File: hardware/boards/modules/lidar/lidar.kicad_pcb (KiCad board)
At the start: 2 copper layers, 70.6 x 66 mm, 33 parts, among them J1 Conn_01x04_Socket, J2 Lidar, J3 Conn_01x03_Socket, J4 Conn_01x03_Socket, J5 Conn_01x03_Socket, J6 Conn_01x03_Socket, J7 Conn_01x05_Socket, J8 Conn_01x04_Socket, Q1 AO3401A, SW1 SW_Push, U1 ATmega128A-A, U2 BNO055, Y1 8MHz, Y2 32.768kHz

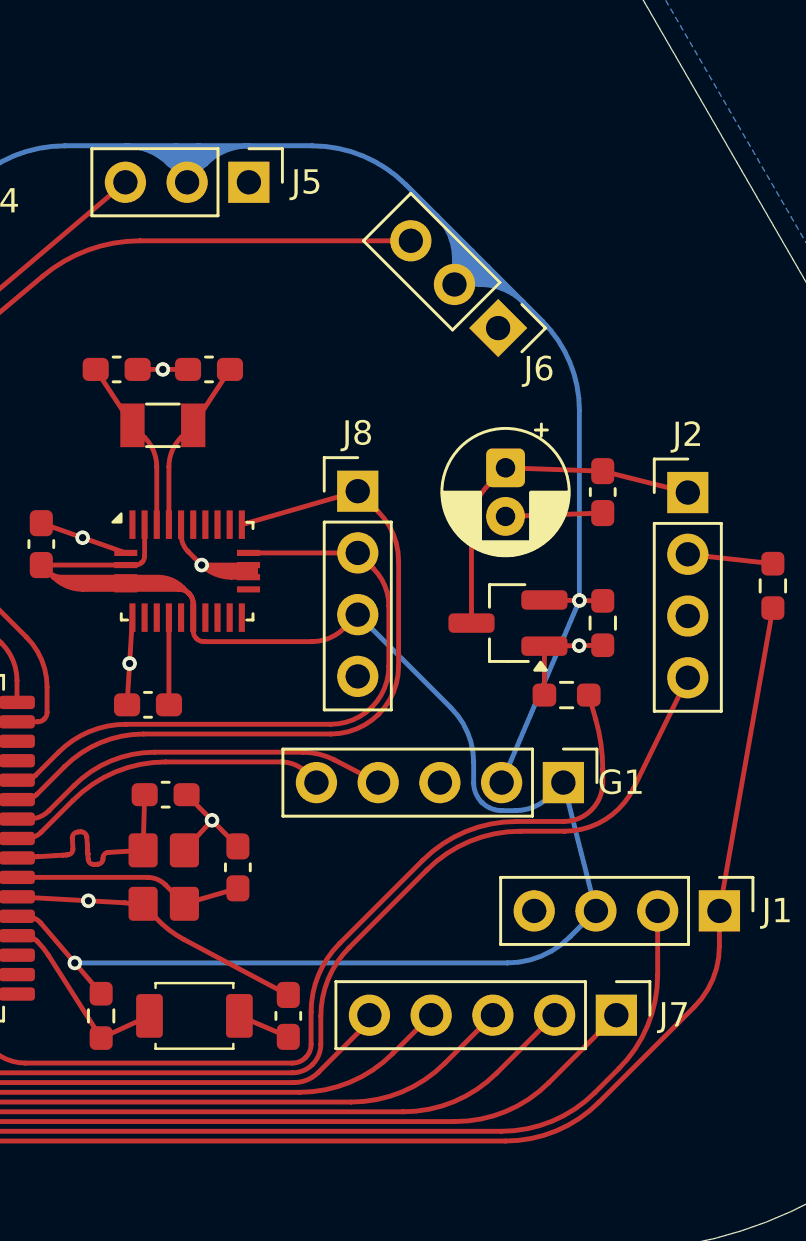
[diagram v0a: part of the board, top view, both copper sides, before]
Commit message: REFACTO relinked every kicad projects
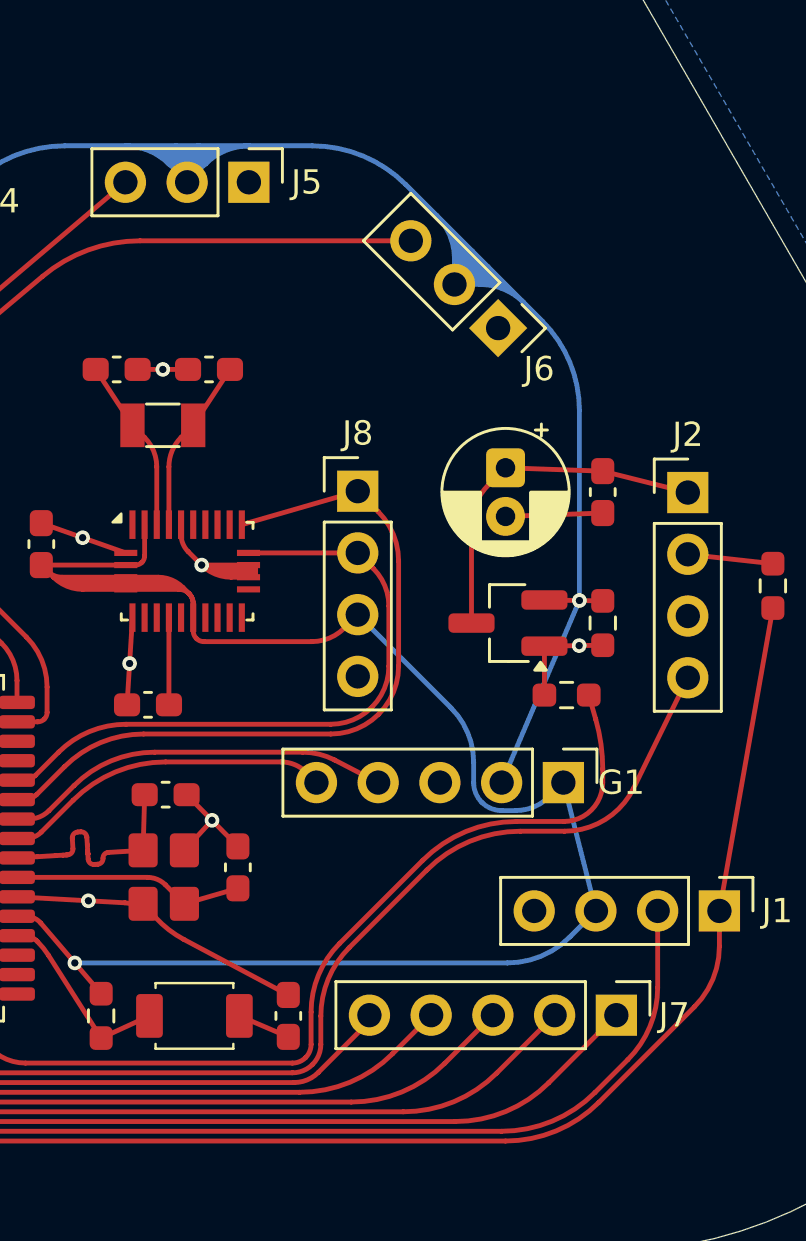
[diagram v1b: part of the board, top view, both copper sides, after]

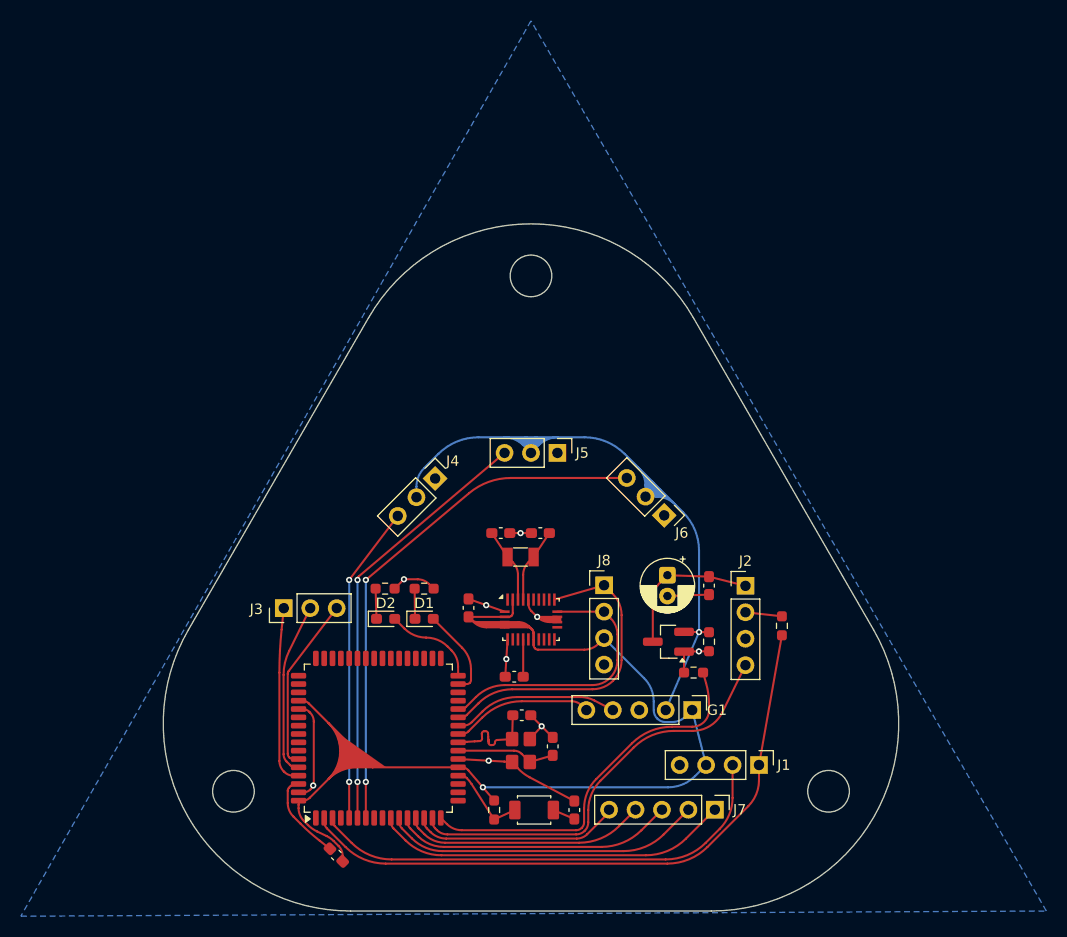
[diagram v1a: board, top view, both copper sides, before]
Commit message: lidar PCB
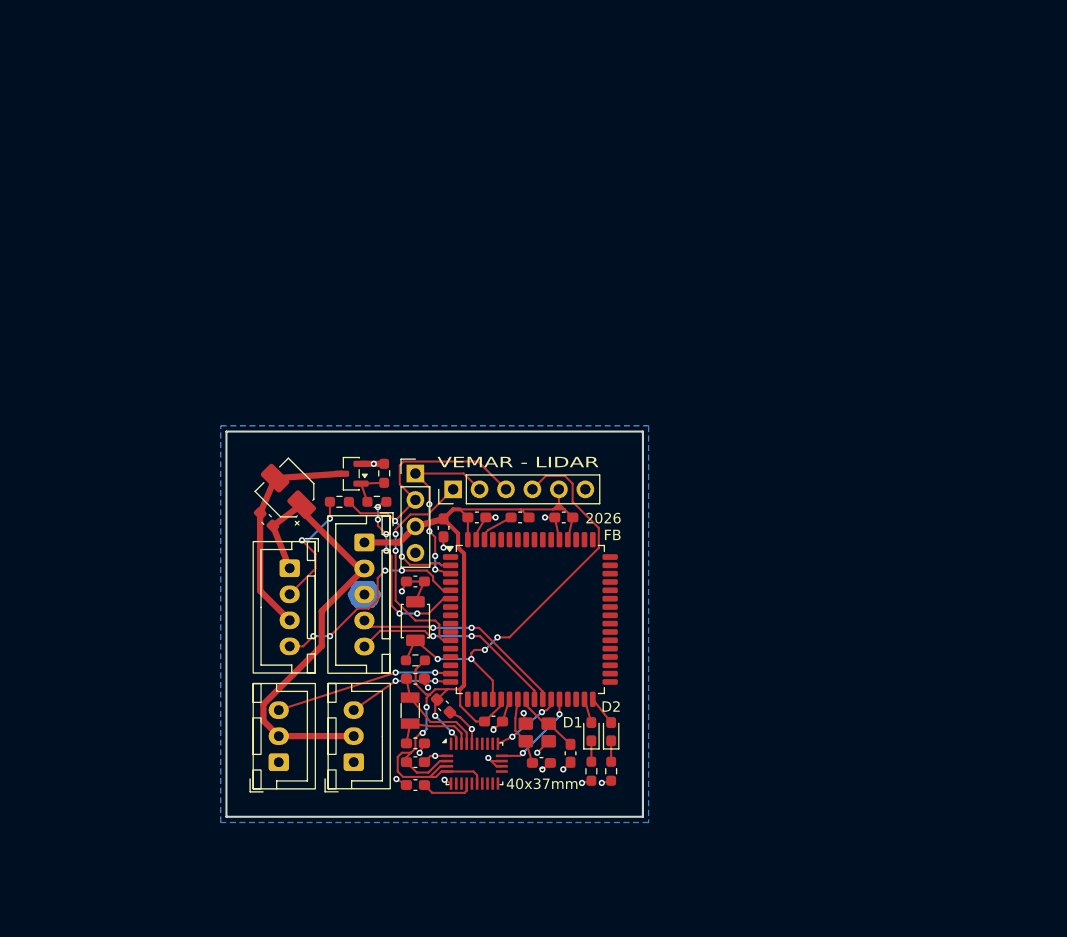
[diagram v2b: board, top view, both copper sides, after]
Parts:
- removed G1: ~, Connector_PinHeader_2.54mm:PinHeader_1x05_P2.54mm_Vertical
- removed J7: Conn_01x05_Socket, Connector_PinHeader_2.54mm:PinHeader_1x05_P2.54mm_Vertical
- removed J8: Conn_01x04_Socket, Connector_PinHeader_2.54mm:PinHeader_1x04_P2.54mm_Vertical
- added C11: 12pF, Capacitor_SMD:C_0603_1608Metric_Pad1.08x0.95mm_HandSolder, F.Cu at (138.9, 105.7)
- added C12: 12pF, Capacitor_SMD:C_0603_1608Metric_Pad1.08x0.95mm_HandSolder, F.Cu at (138.9, 111.9)
- added C13: 100nF, Capacitor_SMD:C_0603_1608Metric_Pad1.08x0.95mm_HandSolder, F.Cu at (138.9, 113.7)
- added C14: 100nF, Capacitor_SMD:C_0603_1608Metric_Pad1.08x0.95mm_HandSolder, F.Cu at (141.6, 108.3)
- added C15: 1uF, Capacitor_SMD:C_0603_1608Metric_Pad1.08x0.95mm_HandSolder, F.Cu at (138.9, 115.9)
- C10: value 12pF -> 100nF
- C4: value 100nF -> 4.7uF
- C5: value 10uF -> 100nF; footprint Capacitor_THT:CP_Radial_D5.0mm_P2.00mm -> Capacitor_SMD:C_0603_1608Metric_Pad1.08x0.95mm_HandSolder
- C7, C8: value 0.1uF -> 100nF
- C9: value 12pF -> 10uF; footprint Capacitor_SMD:C_0603_1608Metric_Pad1.08x0.95mm_HandSolder -> Capacitor_SMD:CP_Elec_4x5.4
- D1: value LED -> GREEN
- D2: value LED -> RED
- J1: value Conn_01x04_Socket -> JST; footprint Connector_PinHeader_2.54mm:PinHeader_1x04_P2.54mm_Vertical -> Connector_JST:JST_XH_B5B-XH-A_1x05_P2.50mm_Vertical
- J2: value Lidar -> Dupont; footprint Connector_PinHeader_2.54mm:PinHeader_1x04_P2.54mm_Vertical -> Connector_PinHeader_2.54mm:PinHeader_1x06_P2.54mm_Vertical
- J3: value Conn_01x03_Socket -> Dupont; footprint Connector_PinHeader_2.54mm:PinHeader_1x03_P2.54mm_Vertical -> Connector_PinHeader_2.54mm:PinHeader_1x04_P2.54mm_Vertical
- J4: value Conn_01x03_Socket -> JST; footprint Connector_PinHeader_2.54mm:PinHeader_1x03_P2.54mm_Vertical -> Connector_JST:JST_XH_B4B-XH-A_1x04_P2.50mm_Vertical
- J5, J6: value Conn_01x03_Socket -> JST; footprint Connector_PinHeader_2.54mm:PinHeader_1x03_P2.54mm_Vertical -> Connector_JST:JST_XH_B3B-XH-A_1x03_P2.50mm_Vertical
- Q1: value AO3401A -> AO3400A; footprint Package_TO_SOT_SMD:SOT-23_Handsoldering -> Package_TO_SOT_SMD:SOT-23
- R4: value 10K -> 100
- R5: value 100 -> 10K
- U1: value ATmega128A-A -> ATmega128A
- Y1: value 8MHz -> 16MHz
- moved R6 44.1 mm to (131.6, 88.7), turned to 180 degrees
- moved J1 43.5 mm to (134.0, 92.6)
- moved J5 40.0 mm to (125.8, 113.7), turned to 90 degrees
- moved J6 38.1 mm to (133.0, 113.7), turned to 90 degrees
- moved R5 35.3 mm to (135.9, 86.0), turned to -90 degrees
- moved R4 34.6 mm to (135.2, 88.7), turned to 180 degrees
- moved Q1 34.5 mm to (132.7, 86.0)
- moved C4 33.1 mm to (141.6, 91.2), turned to -90 degrees
- moved J2 29.6 mm to (142.5, 87.5), turned to 90 degrees
- moved R3 27.9 mm to (157.7, 114.6), turned to -90 degrees
- moved C1 26.7 mm to (138.9, 96.3), turned to 0 degrees
- moved C9 24.5 mm to (126.7, 87.7), turned to 135 degrees
- moved D2 24.2 mm to (157.7, 110.8), turned to 90 degrees
- moved R2 23.8 mm to (155.8, 114.6), turned to -90 degrees
- moved C10 22.5 mm to (124.6, 90.4), turned to 135 degrees
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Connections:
- C1 pad 2: Net-(C1-Pad2) -> GND
- C10 pad 1: Net-(U2-XIN32) -> 5V
- C10 pad 2: GND -> Net-(J4-Pin_3)
- C4 pad 2: Net-(U1-AREF) -> GND
- C5 pad 1: Net-(J2-Pin_1) -> 3V3
- C6 pad 1: Net-(J2-Pin_1) -> 3V3
- C7 pad 1: Net-(U2-CAP) -> 3V3
- C8 pad 1: GND -> 3V3
- C8 pad 2: 3V3 -> Net-(U1-AREF)
- C9 pad 1: Net-(U2-XOUT32) -> 5V
- C9 pad 2: GND -> Net-(J4-Pin_3)
- J1 pad 1: RX0 -> 3V3
- J1 pad 2: TX0 -> 5V
- J1 pad 3: 3V3 -> GND
- J1 pad 4: GND -> SDA
- J2 pad 1: Net-(J2-Pin_1) -> SCK
- J2 pad 2: Net-(J2-Pin_2) -> TX0
- J2 pad 3: GND -> RX0
- J2 pad 4: LIDAR_PWM -> RST
- J3 pad 1: ADC0 -> TX0
- J3 pad 2: ADC1 -> RX0
- J3 pad 3: ADC2 -> 3V3
- J4 pad 1: GND -> 5V
- J4 pad 2: 5V -> Net-(J4-Pin_2)
- J4 pad 3: SERVO_A_PWM -> Net-(J4-Pin_3)
- J5 pad 3: SERVO_B_PWM -> SERVO_A_PWM
- J6 pad 3: SERVO_C_PWM -> SERVO_B_PWM
- Q1 pad 1: GND -> Net-(Q1-G)
- Q1 pad 2: 5V -> GND
- Q1 pad 3: Net-(J2-Pin_1) -> Net-(J4-Pin_3)
- R4 pad 1: GND -> LIDAR_EN
- R4 pad 2: 5V -> Net-(Q1-G)
- R5 pad 1: LIDAR_EN -> GND
- R5 pad 2: GND -> Net-(Q1-G)
- R6 pad 2: Net-(J2-Pin_2) -> Net-(J4-Pin_2)
- SW1 pad 1: Net-(C1-Pad2) -> GND
- U1 pad 10: DEBUG_0 -> unconnected-(U1-PB0-Pad10)
- U1 pad 11: DEBUG_1 -> SCK
- U1 pad 12: DEBUG_2 -> unconnected-(U1-PB2-Pad12)
- U1 pad 13: DEBUG_3 -> unconnected-(U1-PB3-Pad13)
- U1 pad 14: DEBUG_4 -> unconnected-(U1-PB4-Pad14)
- U1 pad 15: LIDAR_PWM -> SERVO_A_PWM
- U1 pad 16: LIDAR_EN -> SERVO_B_PWM
- U1 pad 5: SERVO_A_PWM -> LIDAR_PWM
- U1 pad 59: ADC2 -> unconnected-(U1-PF2-Pad59)
- U1 pad 6: SERVO_B_PWM -> LIDAR_EN
- U1 pad 60: ADC1 -> unconnected-(U1-PF1-Pad60)
- U1 pad 61: ADC0 -> unconnected-(U1-PF0-Pad61)
- U1 pad 7: SERVO_C_PWM -> unconnected-(U1-PE5-Pad7)
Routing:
- net SERVO_C_PWM: track 51.3 -> 0.00 mm, vias 2 -> 0
- net DEBUG_0: track 34.3 -> 0.00 mm
- net RST: track 7.86 -> 41.8 mm, vias 0 -> 4
- net SERVO_B_PWM: track 41.6 -> 10.2 mm
- net DEBUG_1: track 30.7 -> 0.00 mm
- net RX0: track 61.6 -> 32.3 mm, vias 0 -> 2
- net TX0: track 46.3 -> 18.3 mm, vias 0 -> 4
- net DEBUG_2: track 27.0 -> 0.00 mm
- net 5V: track 69.5 -> 44.7 mm, vias 1 -> 0
- net RX1: track 30.9 -> 6.95 mm, vias 0 -> 2
- net DEBUG_3: track 23.4 -> 0.00 mm
- net Net-(J4-Pin_3): track 0.00 -> 21.5 mm
- net SCK: track 0.00 -> 21.5 mm, vias 0 -> 2
- net DEBUG_4: track 20.1 -> 0.00 mm
- net LIDAR_PWM: track 40.0 -> 20.7 mm, vias 0 -> 4
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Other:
- board size 70.6 x 66 mm -> 40 x 37 mm
- board text added: "2026 FB"
- board text added: "40x37mm"
- board text added: "A"
- board text added: "B"
- board text added: "I2C"
- board text added: "ISP"
- board text added: "LIDAR"
- board text added: "SERVOS"
- board text added: "UART"
- board text added: "VEMAR - LIDAR"
